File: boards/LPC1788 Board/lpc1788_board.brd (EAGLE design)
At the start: 81.8 x 67.7 mm, 99 parts, among them J1 5VDC, J10 MOLEX_527930570_5PIN_FFC_CONN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, J11 20PIN_10X2_.100IN, J12 DF12B-50DX_25X2_0.5MM, J2 SAMTEC_MUSB, J3 JST_2MM_SMT, J4 Console, J5 SMA-J-P-X-ST-EM1, J6 JTAG, J8 NHD-4.3-480272EF, J9 DF12B-50DX_25X2_0.5MM, Q1 MMBT2907, SW1 Reset, SW2 OS102011MA1QS1, U1 LTC3127EMSEPBF, U2 MAX1551EZK+T, U3 LT3497EDDBTRMPBF, U4 CY62167_16MBIT_SRAM, U5 S25FL064P, U6 AR1021-RESISTIVE_TOUCH_CONTRO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, Y1 12MHz

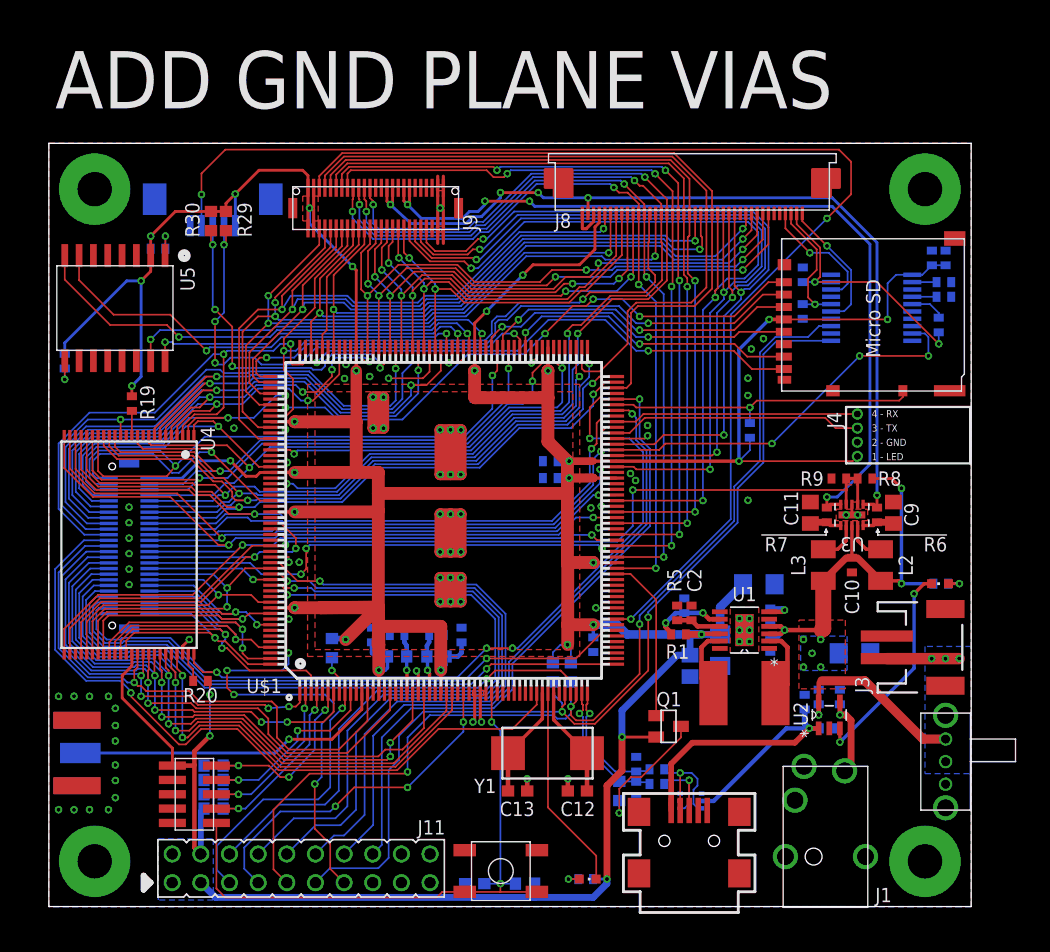
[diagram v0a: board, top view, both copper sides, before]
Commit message: updates
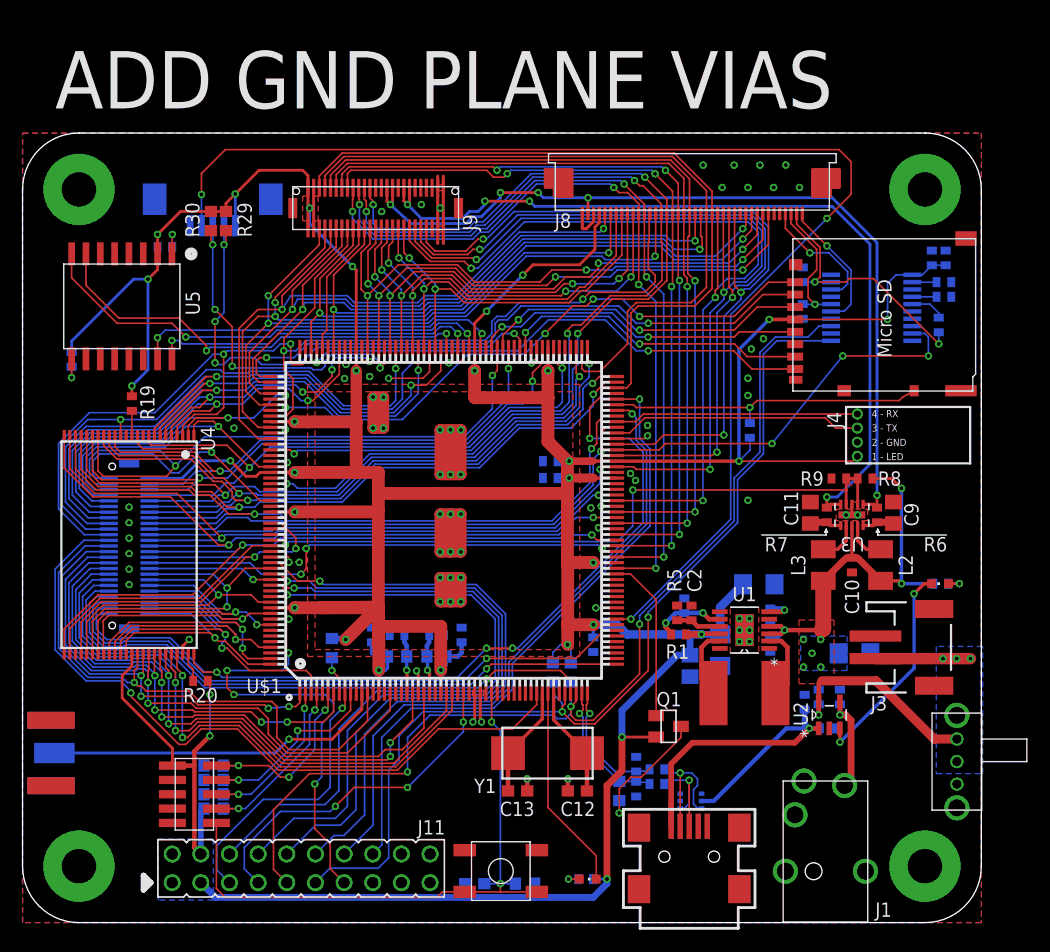
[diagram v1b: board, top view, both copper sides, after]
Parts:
- moved J5 2.30 mm to (-47.6, 53.0)
- moved J2 1.40 mm to (11.1, 38.0)
- moved J1 1.30 mm to (23.9, 47.6)
- moved J3 1.00 mm to (30.0, 62.4)
- moved SW2 1.00 mm to (34.8, 52.3)
- moved U$3 1.00 mm to (27.1, 91.9)
- moved R22 0.63 mm to (-43.6, 87.9)
- moved R28 0.63 mm to (-35.4, 97.9)
- moved U5 0.63 mm to (-39.2, 92.6)
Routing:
- net +VUSB: track 34.2 -> 37.0 mm
- net N$27: track 28.0 -> 30.3 mm
- net N$20: track 6.42 -> 8.42 mm
- net D_P: track 8.08 -> 9.48 mm
- net D_N: track 10.0 -> 11.4 mm
- net V+: track 8.04 -> 9.34 mm
- net SD_DAT_3: track 53.6 -> 54.6 mm
- net SD_DAT_2: track 52.3 -> 53.3 mm
- net SD_DAT_0: track 26.3 -> 27.3 mm
- net SD_CMD: track 28.6 -> 29.6 mm
- net SD_CLK: track 28.8 -> 29.8 mm
- net +VBAT: track 55.4 -> 56.4 mm
- net SD_DAT_1: track 46.1 -> 47.1 mm
- net SPI_FLASH_MOSI: track 33.8 -> 33.1 mm
- net SD_DET: track 27.8 -> 28.4 mm
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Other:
- board size 81.8 x 67.7 mm -> 85 x 70 mm
- board text added: "Ryan Mamone 2014"
- board text removed: "Ryan Mamonw 2014"
